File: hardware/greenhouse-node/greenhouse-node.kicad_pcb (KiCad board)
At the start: 2 copper layers, 90.2 x 69.8 mm, 49 parts, among them J1 Conn_01x12_Male, J2 Conn_01x02_Male, J3 Conn_01x02_Male, J4 Conn_01x02_Male, J5 Conn_01x04_Male, J6 RX_PinHeader_1x04_P2.54mm, J7 TX_PinHeader_1x04_P2.54mm, J8 Conn_01x02_Male, Q1 BC549C, Q2 BC549C, Q3 BC549C, Q4 IRF9530N, Q5 IRF530N, Q6 IRF9530N, Q7 IRF530N, Q8 BC549C, Q9 BC549C, U1 ATtiny84A-P, U2 L7805, U3 74HC595

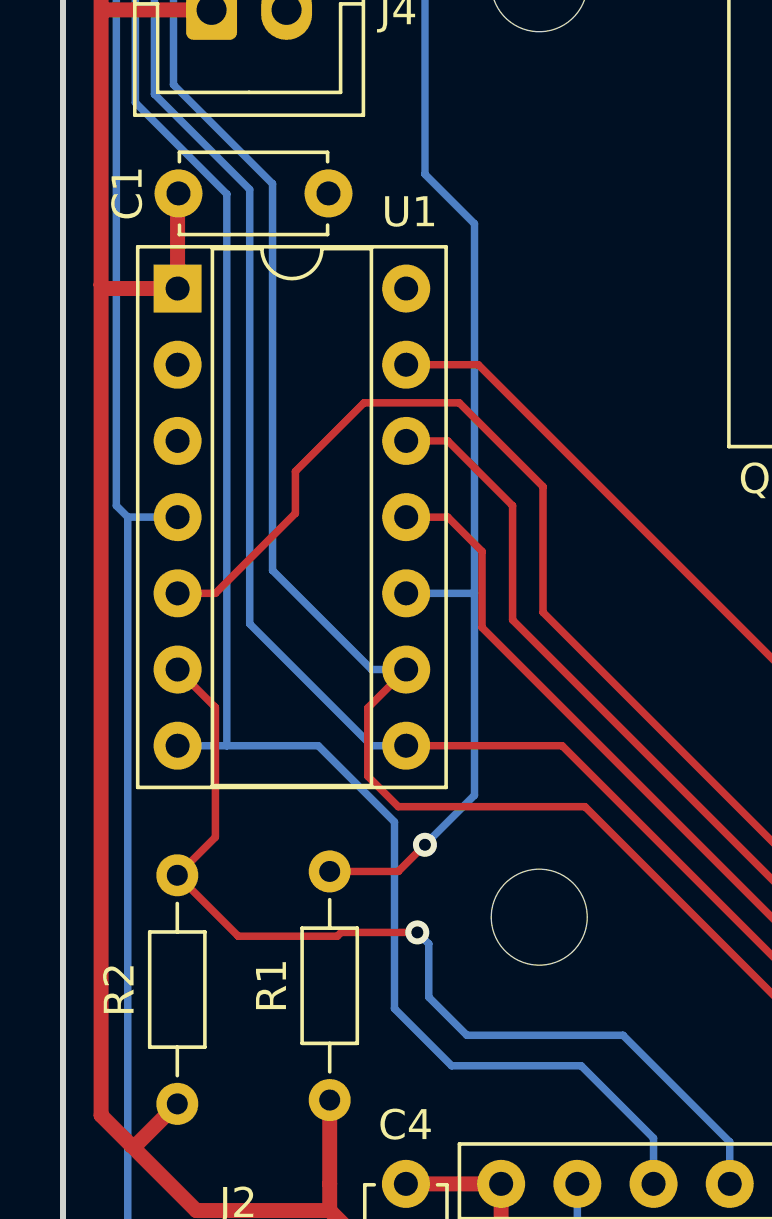
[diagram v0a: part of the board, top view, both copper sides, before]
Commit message: Tweak net positions
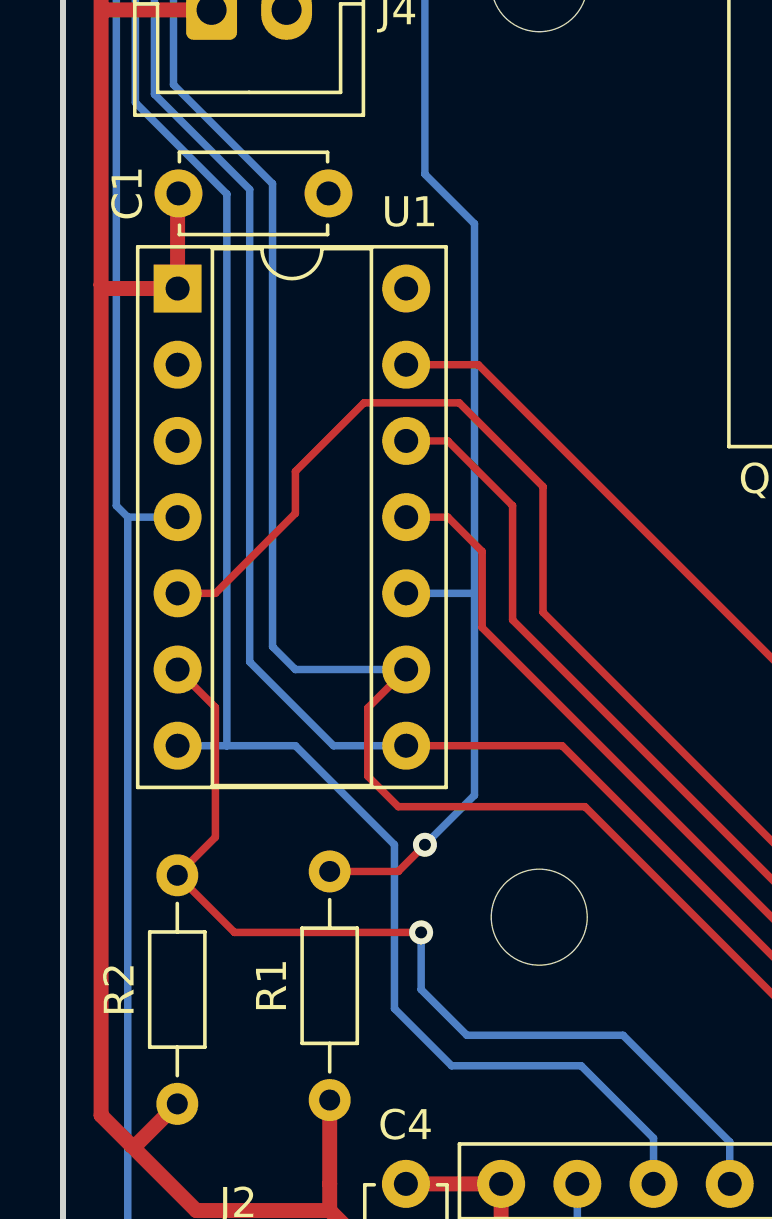
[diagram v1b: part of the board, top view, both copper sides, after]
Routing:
- net /SR_RCLK: track 66.9 -> 68.4 mm
- net /SR_CLK: track 64.8 -> 65.6 mm
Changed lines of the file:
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@@
   (segment (start 139.446 92.837) (end 138.43 91.821) (width 0.25) (layer "F.Cu") (net 13))
   (segment (start 145.669 92.837) (end 139.446 92.837) (width 0.25) (layer "F.Cu") (net 13))
+  (segment (start 135.255 87.503) (end 135.255 72.0725) (width 0.25) (layer "B.Cu") (net 13))
+  (segment (start 134.511254 62.738) (end 137.541 62.738) (width 0.25) (layer "B.Cu") (net 13))
+  (segment (start 136.017 88.265) (end 135.255 87.503) (width 0.25) (layer "B.Cu") (net 13))
+  (segment (start 131.953 65.296254) (end 134.511254 62.738) (width 0.25) (layer "B.Cu") (net 13))
+  (segment (start 139.71 88.265) (end 136.017 88.265) (width 0.25) (layer "B.Cu") (net 13))
+  (segment (start 137.541 62.738) (end 140.723 59.556) (width 0.25) (layer "B.Cu") (net 13))
+  (segment (start 131.953 68.7705) (end 131.953 65.296254) (width 0.25) (layer "B.Cu") (net 13))
+  (segment (start 140.723 59.556) (end 140.723 58.022) (width 0.25) (layer "B.Cu") (net 13))
   (segment (start 135.255 72.0725) (end 131.953 68.7705) (width 0.25) (layer "B.Cu") (net 13))
-  (segment (start 131.953 65.296254) (end 134.511254 62.738) (width 0.25) (layer "B.Cu") (net 13))
-  (segment (start 137.541 62.738) (end 140.723 59.556) (width 0.25) (layer "B.Cu") (net 13))
-  (segment (start 138.557 88.265) (end 135.255 84.963) (width 0.25) (layer "B.Cu") (net 13))
-  (segment (start 131.953 68.7705) (end 131.953 65.296254) (width 0.25) (layer "B.Cu") (net 13))
-  (segment (start 135.255 84.963) (end 135.255 72.0725) (width 0.25) (layer "B.Cu") (net 13))
-  (segment (start 139.71 88.265) (end 138.557 88.265) (width 0.25) (layer "B.Cu") (net 13))
-  (segment (start 134.511254 62.738) (end 137.541 62.738) (width 0.25) (layer "B.Cu") (net 13))
-  (segment (start 140.723 59.556) (end 140.723 58.022) (width 0.25) (layer "B.Cu") (net 13))
+  (segment (start 139.319 94.107) (end 139.319 99.568) (width 0.25) (layer "B.Cu") (net 14))
+  (segment (start 132.09 90.805) (end 133.731 90.805) (width 0.25) (layer "B.Cu") (net 14))
+  (segment (start 145.542 101.473) (end 147.955 103.886) (width 0.25) (layer "B.Cu") (net 14))
   (segment (start 147.955 103.886) (end 147.955 105.41) (width 0.25) (layer "B.Cu") (net 14))
-  (segment (start 132.09 90.805) (end 133.731 90.805) (width 0.25) (layer "B.Cu") (net 14))
-  (segment (start 141.224 101.473) (end 145.542 101.473) (width 0.25) (layer "B.Cu") (net 14))
   (segment (start 135.723 59.476) (end 135.723 58.022) (width 0.25) (layer "B.Cu") (net 14))
-  (segment (start 133.731 90.805) (end 136.779 90.805) (width 0.25) (layer "B.Cu") (net 14))
   (segment (start 139.319 99.568) (end 141.224 101.473) (width 0.25) (layer "B.Cu") (net 14))
   (segment (start 130.683 64.516) (end 135.723 59.476) (width 0.25) (layer "B.Cu") (net 14))
   (segment (start 133.731 90.805) (end 133.731 72.415701) (width 0.25) (layer "B.Cu") (net 14))
   (segment (start 133.731 72.415701) (end 130.683 69.367701) (width 0.25) (layer "B.Cu") (net 14))
+  (segment (start 133.731 90.805) (end 136.017 90.805) (width 0.25) (layer "B.Cu") (net 14))
   (segment (start 130.683 69.367701) (end 130.683 64.516) (width 0.25) (layer "B.Cu") (net 14))
-  (segment (start 139.319 93.345) (end 139.319 99.568) (width 0.25) (layer "B.Cu") (net 14))
-  (segment (start 145.542 101.473) (end 147.955 103.886) (width 0.25) (layer "B.Cu") (net 14))
-  (segment (start 136.779 90.805) (end 139.319 93.345) (width 0.25) (layer "B.Cu") (net 14))
+  (segment (start 136.017 90.805) (end 139.319 94.107) (width 0.25) (layer "B.Cu") (net 14))
+  (segment (start 141.224 101.473) (end 145.542 101.473) (width 0.25) (layer "B.Cu") (net 14))
   (segment (start 144.907 90.805) (end 155.575 101.473) (width 0.25) (layer "F.Cu") (net 15))
   (segment (start 155.575 101.473) (end 155.575 105.41) (width 0.25) (layer "F.Cu") (net 15))
   (segment (start 139.71 90.805) (end 144.907 90.805) (width 0.25) (layer "F.Cu") (net 15))
+  (segment (start 134.493 72.263) (end 131.318 69.088) (width 0.25) (layer "B.Cu") (net 15))
+  (segment (start 138.223 59.389) (end 138.223 58.022) (width 0.25) (layer "B.Cu") (net 15))
+  (segment (start 131.318 69.088) (end 131.318 64.897) (width 0.25) (layer "B.Cu") (net 15))
+  (segment (start 131.318 64.897) (end 134.493 61.722) (width 0.25) (layer "B.Cu") (net 15))
   (segment (start 135.89 61.722) (end 138.223 59.389) (width 0.25) (layer "B.Cu") (net 15))
-  (segment (start 131.318 69.088) (end 131.318 64.897) (width 0.25) (layer "B.Cu") (net 15))
-  (segment (start 134.493 72.263) (end 131.318 69.088) (width 0.25) (layer "B.Cu") (net 15))
-  (segment (start 131.318 64.897) (end 134.493 61.722) (width 0.25) (layer "B.Cu") (net 15))
-  (segment (start 139.71 90.805) (end 138.557 90.805) (width 0.25) (layer "B.Cu") (net 15))
-  (segment (start 138.557 90.805) (end 134.493 86.741) (width 0.25) (layer "B.Cu") (net 15))
   (segment (start 134.493 61.722) (end 135.89 61.722) (width 0.25) (layer "B.Cu") (net 15))
-  (segment (start 134.493 86.741) (end 134.493 72.263) (width 0.25) (layer "B.Cu") (net 15))
-  (segment (start 138.223 59.389) (end 138.223 58.022) (width 0.25) (layer "B.Cu") (net 15))
+  (segment (start 137.287 90.805) (end 134.493 88.011) (width 0.25) (layer "B.Cu") (net 15))
+  (segment (start 139.71 90.805) (end 137.287 90.805) (width 0.25) (layer "B.Cu") (net 15))
+  (segment (start 134.493 88.011) (end 134.493 72.263) (width 0.25) (layer "B.Cu") (net 15))
   (segment (start 132.08 95.123) (end 133.35 93.853) (width 0.25) (layer "F.Cu") (net 16))
   (segment (start 133.35 93.853) (end 133.35 89.525) (width 0.25) (layer "F.Cu") (net 16))
+  (segment (start 140.208 97.028) (end 133.985 97.028) (width 0.25) (layer "F.Cu") (net 16))
+  (segment (start 133.985 97.028) (end 132.08 95.123) (width 0.25) (layer "F.Cu") (net 16))
   (segment (start 133.35 89.525) (end 132.09 88.265) (width 0.25) (layer "F.Cu") (net 16))
-  (segment (start 134.112 97.155) (end 132.08 95.123) (width 0.25) (layer "F.Cu") (net 16))
-  (segment (start 137.414 97.155) (end 134.112 97.155) (width 0.25) (layer "F.Cu") (net 16))
-  (segment (start 140.081 97.028) (end 137.541 97.028) (width 0.25) (layer "F.Cu") (net 16))
-  (segment (start 137.541 97.028) (end 137.414 97.155) (width 0.25) (layer "F.Cu") (net 16))
-  (via (at 140.081 97.028) (size 0.8) (drill 0.4) (layers "F.Cu" "B.Cu") (net 16))
+  (via (at 140.208 97.028) (size 0.8) (drill 0.4) (layers "F.Cu" "B.Cu") (net 16))
+  (segment (start 146.939 100.457) (end 150.495 104.013) (width 0.25) (layer "B.Cu") (net 16))
+  (segment (start 140.208 98.933) (end 141.732 100.457) (width 0.25) (layer "B.Cu") (net 16))
   (segment (start 141.732 100.457) (end 146.939 100.457) (width 0.25) (layer "B.Cu") (net 16))
-  (segment (start 140.081 97.028) (end 140.462 97.409) (width 0.25) (layer "B.Cu") (net 16))
-  (segment (start 140.462 99.187) (end 141.732 100.457) (width 0.25) (layer "B.Cu") (net 16))
-  (segment (start 140.462 97.409) (end 140.462 99.187) (width 0.25) (layer "B.Cu") (net 16))
+  (segment (start 140.208 97.028) (end 140.208 98.933) (width 0.25) (layer "B.Cu") (net 16))
   (segment (start 150.495 104.013) (end 150.495 105.41) (width 0.25) (layer "B.Cu") (net 16))
-  (segment (start 146.939 100.457) (end 150.495 104.013) (width 0.25) (layer "B.Cu") (net 16))
   (segment (start 139.446 94.996) (end 137.16 94.996) (width 0.25) (layer "F.Cu") (net 17))
   (segment (start 140.335 94.107) (end 139.446 94.996) (width 0.25) (layer "F.Cu") (net 17))
